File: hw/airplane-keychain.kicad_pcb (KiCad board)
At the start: 2 copper layers, 103.1 x 141.7 mm, 19 parts, among them IC1 ATTINY85-P, J1 CONN_01X03_MALE, SW1 SW_PUSH, SW2 SPST

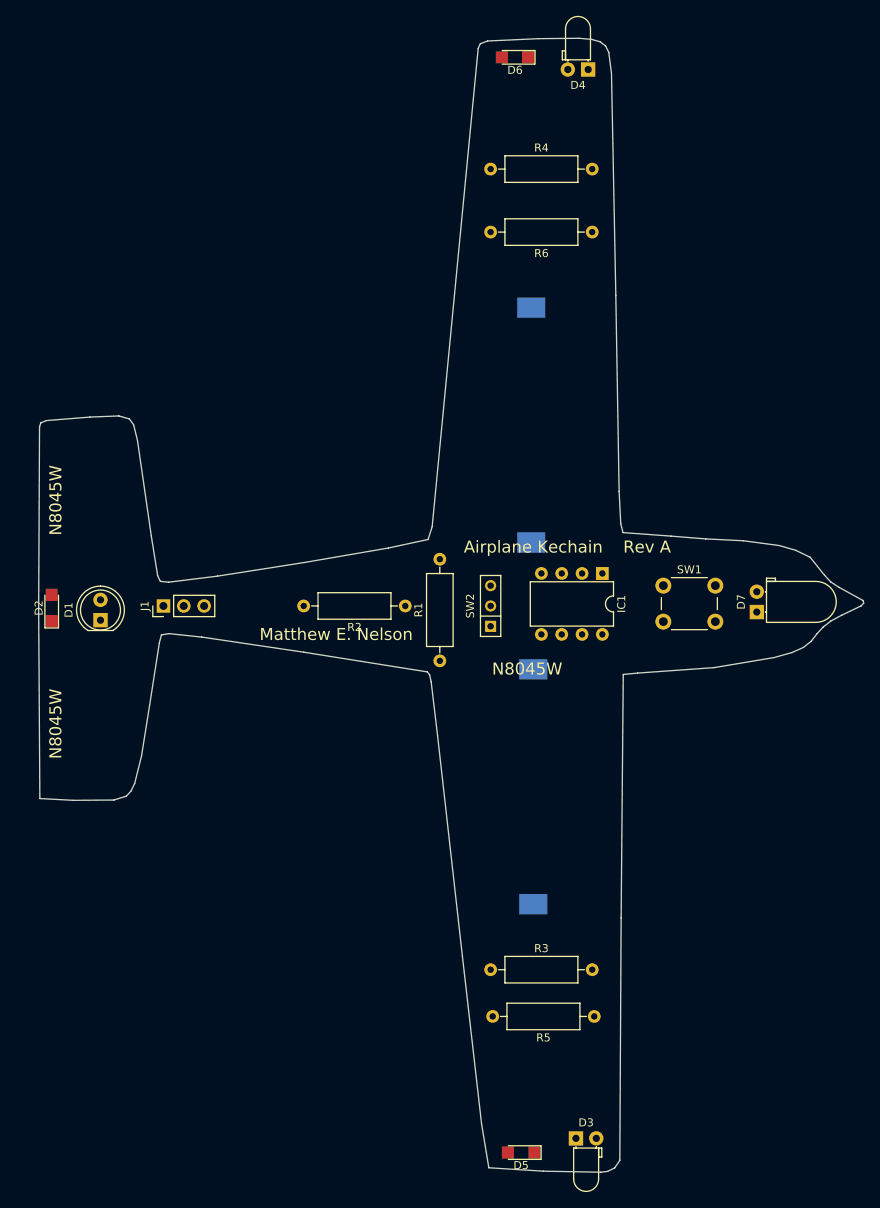
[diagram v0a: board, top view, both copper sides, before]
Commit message: Initial update for ISGC model
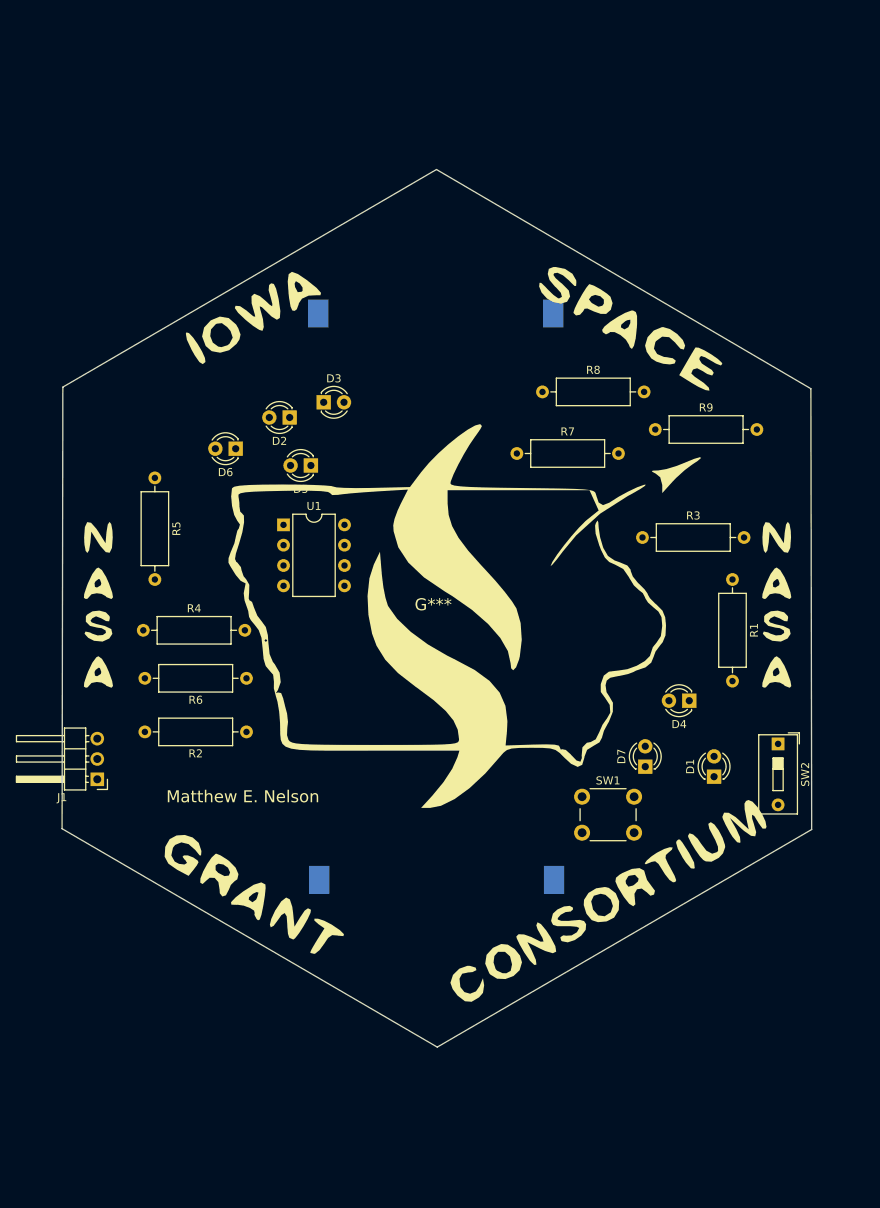
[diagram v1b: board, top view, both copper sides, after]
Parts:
- removed IC1: ATTINY85-P, Housings_DIP:DIP-8_W7.62mm
- added G***: LOGO, LOGO, F.Cu at (130.5, 95.6)
- added R7: 100, Resistor_THT:R_Axial_DIN0309_L9.0mm_D3.2mm_P12.70mm_Horizontal, F.Cu at (140.9, 76.7)
- added R8: 100, Resistor_THT:R_Axial_DIN0309_L9.0mm_D3.2mm_P12.70mm_Horizontal, F.Cu at (144.2, 69.0)
- added R9: 100, Resistor_THT:R_Axial_DIN0309_L9.0mm_D3.2mm_P12.70mm_Horizontal, F.Cu at (158.2, 73.7)
- added U1: ATtiny85-20P, Package_DIP:DIP-8_W7.62mm, F.Cu at (111.8, 85.6)
- BT1, BT2: footprint Battery_Holders:Keystone_1058_1x2032-CoinCell -> Battery:BatteryHolder_Keystone_1058_1x2032
- D1: footprint LEDs:LED_D5.0mm -> LED_THT:LED_D3.0mm
- D2, D5, D6: footprint LEDs:LED_1206 -> LED_THT:LED_D3.0mm
- D3, D4: footprint LEDs:LED_D3.0mm_Horizontal_O1.27mm_Z2.0mm -> LED_THT:LED_D3.0mm
- D7: footprint LEDs:LED_D5.0mm_Horizontal_O1.27mm_Z3.0mm -> LED_THT:LED_D3.0mm
- J1: footprint Pin_Headers:Pin_Header_Straight_1x03_Pitch2.54mm -> Connector_PinHeader_2.54mm:PinHeader_1x03_P2.54mm_Horizontal
- R1, R2, R3, R4, R5, R6: footprint Resistors_THT:R_Axial_DIN0309_L9.0mm_D3.2mm_P12.70mm_Horizontal -> Resistor_THT:R_Axial_DIN0309_L9.0mm_D3.2mm_P12.70mm_Horizontal
- SW1: footprint Buttons_Switches_THT:SW_PUSH_6mm -> Button_Switch_THT:SW_PUSH_6mm
- SW2: footprint Buttons_Switches_THT:SW_Micro_SPST -> Button_Switch_THT:SW_DIP_SPSTx01_Slide_9.78x4.72mm_W7.62mm_P2.54mm
- moved D3 97.3 mm to (116.8, 70.3)
- moved D5 89.8 mm to (115.2, 78.2)
- moved R5 86.9 mm to (95.7, 79.8), turned to -90 degrees
- moved D4 79.9 mm to (162.5, 107.6)
- moved D1 79.2 mm to (165.6, 117.1)
- moved R4 72.2 mm to (94.2, 98.8)
- moved R6 70.6 mm to (107.2, 104.8)
- moved D6 60.1 mm to (105.8, 76.1)
- moved R3 57.3 mm to (156.7, 87.2)
- moved SW2 39.9 mm to (173.6, 113.0), turned to -90 degrees
- moved D2 38.1 mm to (112.5, 72.2), turned to 180 degrees
- moved R1 38.0 mm to (167.9, 92.5), turned to -90 degrees
- moved SW1 28.3 mm to (149.1, 119.6)
- moved R2 25.3 mm to (107.2, 111.5)
- moved D7 23.8 mm to (157.0, 115.8)
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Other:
- board size 103.1 x 141.7 mm -> 93.7 x 109.7 mm
- board text removed: "Airplane Kechain"
- board text removed: "N8045W"
- board text removed: "Rev A"
